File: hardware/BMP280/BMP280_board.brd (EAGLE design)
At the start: 17.6 x 17.6 mm, 8 parts, among them U1 BMP280, U2 EM406FLAT

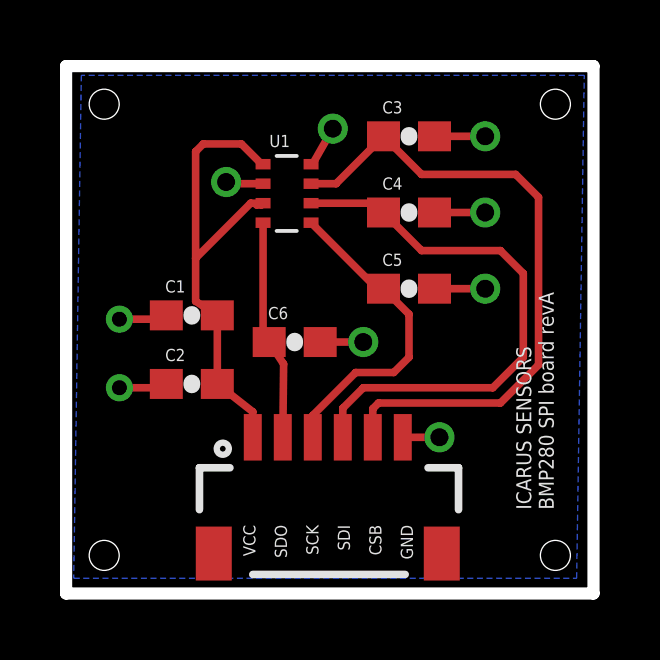
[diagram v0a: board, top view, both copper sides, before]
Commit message: BMP280
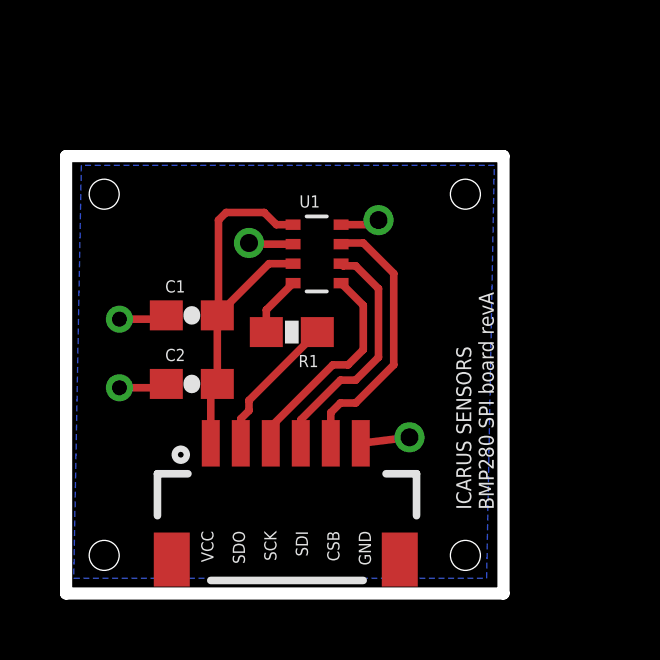
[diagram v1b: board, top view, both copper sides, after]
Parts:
- removed C3, C4, C5, C6: 56pF, SparkFun-Capacitors:0603-CAP
- added R1: (no value), SparkFun-Passives:0603-RES
- C1: value 0.1uF -> 1.0uF
- moved U1 2.25 mm to (8.62, 11.6)
- moved U2 1.41 mm to (7.62, 2.34)
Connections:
- new net N$1: R1.2, U1.5
- net CSB: no longer C3.1
- net GND: no longer C3.2, C4.2, C5.2, C6.2
- net SCK: no longer C5.1
- net SDI: no longer C4.1
- net SDO: now also R1.1; no longer C6.1, U1.5
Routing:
- net CSB: track 21.7 -> 9.02 mm
- net SDI: track 18.5 -> 8.12 mm
- net GND: track 13.8 -> 7.69 mm, vias 9 -> 5
- net SCK: track 10.7 -> 7.22 mm
- net VCC: track 16.8 -> 13.8 mm
- net SDO: track 7.38 -> 4.76 mm
- net N$1: track 0.00 -> 2.00 mm
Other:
- board size 17.6 x 17.6 mm -> 14.6 x 14.6 mm

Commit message: MS5803
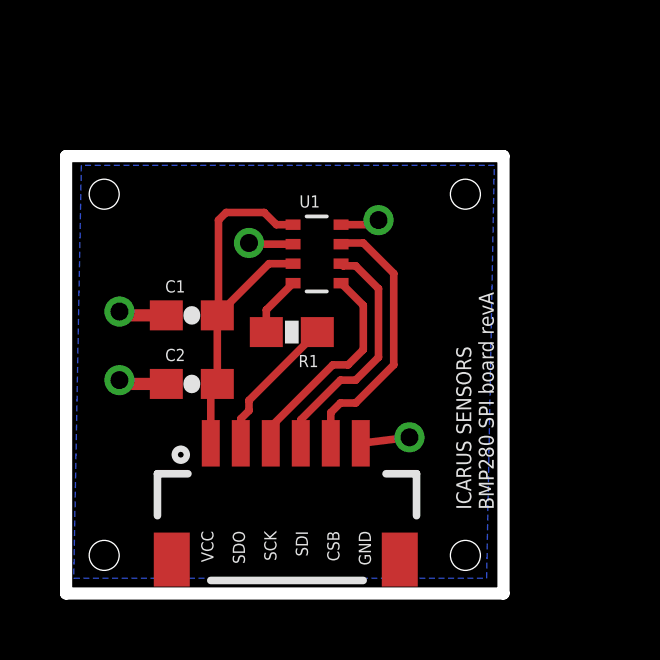
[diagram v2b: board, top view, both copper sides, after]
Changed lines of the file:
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@@
 <contactref element="C1" pad="2"/>
 <contactref element="C2" pad="2"/>
-<via x="2.032" y="9.398" extent="1-16" drill="0.5" diameter="0.254"/>
-<via x="2.032" y="7.112" extent="1-16" drill="0.5" diameter="0.254"/>
-<wire x1="2.032" y1="9.398" x2="3.595" y2="9.398" width="0.254" layer="1"/>
-<wire x1="2.032" y1="7.112" x2="3.595" y2="7.112" width="0.254" layer="1"/>
-<wire x1="3.595" y1="7.112" x2="3.595" y2="7.239" width="0.254" layer="1"/>
 <via x="6.35" y="11.938" extent="1-16" drill="0.6"/>
 <via x="10.668" y="12.7" extent="1-16" drill="0.6"/>
@@
 <wire x1="6.39" y1="11.898" x2="7.82" y2="11.898" width="0.254" layer="1"/>
 <wire x1="9.42" y1="12.548" x2="10.516" y2="12.548" width="0.254" layer="1"/>
-<wire x1="3.595" y1="9.398" x2="3.595" y2="9.525" width="0" layer="19" extent="1-1"/>
+<via x="2.032" y="9.652" extent="1-16" drill="0.6"/>
+<via x="2.032" y="7.366" extent="1-16" drill="0.6"/>
+<wire x1="3.595" y1="7.239" x2="3.595" y2="9.525" width="0" layer="19" extent="1-1"/>
+<wire x1="3.595" y1="9.525" x2="2.159" y2="9.525" width="0.4064" layer="1"/>
+<wire x1="2.159" y1="9.525" x2="2.032" y2="9.652" width="0.4064" layer="1"/>
+<wire x1="3.595" y1="7.239" x2="2.159" y2="7.239" width="0.4064" layer="1"/>
+<wire x1="2.159" y1="7.239" x2="2.032" y2="7.366" width="0.4064" layer="1"/>
 </signal>
 <signal name="CSB">
